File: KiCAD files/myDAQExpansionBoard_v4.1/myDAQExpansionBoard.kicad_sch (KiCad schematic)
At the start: 73 parts, among them J1 Conn_01x05_Male, J2 Conn_01x05_Male, J3 Conn_01x08_Male, J4 OSTV7XX3151, J5 Screw_Terminal_01x02, J6 Screw_Terminal_01x02, J7 Screw_Terminal_01x01, J8 Screw_Terminal_01x01, SW1 SW_SPDT, SW2 SW_SPDT, SW3 SW_Push, SW4 SW_Push, U1 74LS47, U2 7segm-symbol, U3 ACS712xLCTR-05B, U4 L298N

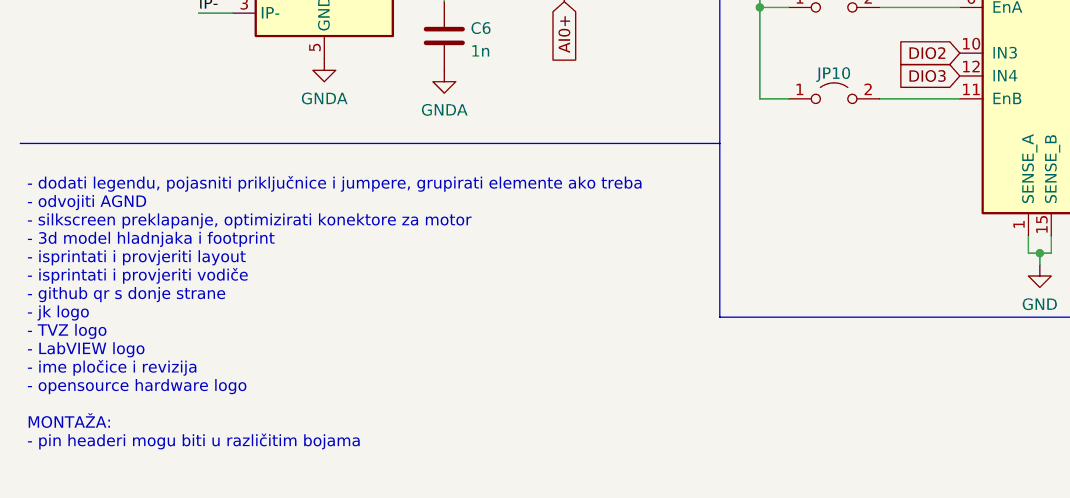
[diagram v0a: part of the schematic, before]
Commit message: update
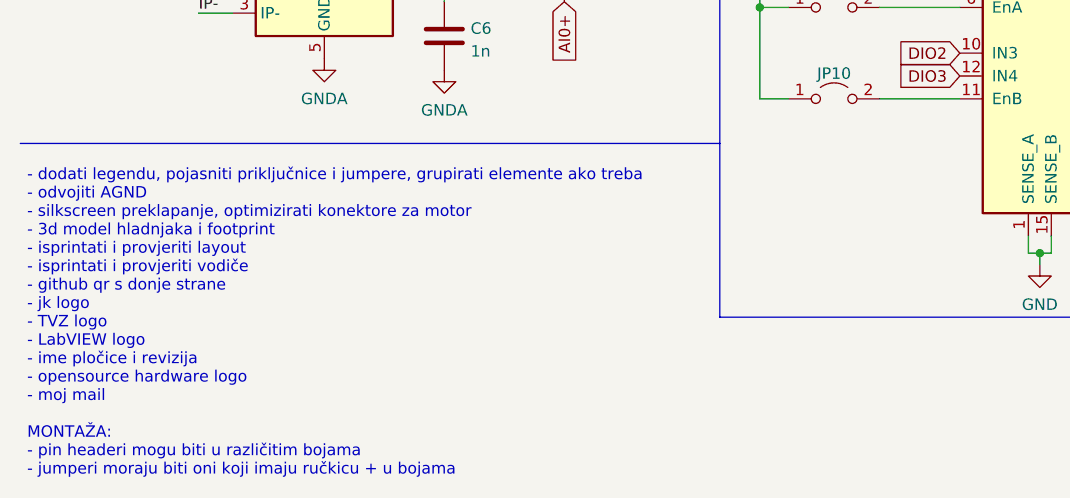
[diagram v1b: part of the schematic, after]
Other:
- note added: "- dodati legendu, pojasniti priključnice i jumpere, grupirati elemente ako treba - odvojiti AGND - silkscreen preklapanje, optimizirati konektore za motor - 3d model hladnjaka i footprint - isprintati i provjeriti layout - isprintati i provjeriti vodiče - github qr s donje strane - jk logo - TVZ logo - LabVIEW logo - ime pločice i revizija - opensource hardware logo - moj mail MONTAŽA: - pin head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"
- note removed: "- dodati legendu, pojasniti priključnice i jumpere, grupirati elemente ako treba - odvojiti AGND - silkscreen preklapanje, optimizirati konektore za motor - 3d model hladnjaka i footprint - isprintati i provjeriti layout - isprintati i provjeriti vodiče - github qr s donje strane - jk logo - TVZ logo - LabVIEW logo - ime pločice i revizija - opensource hardware logo MONTAŽA: - pin headeri mogu bi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"
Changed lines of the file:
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@@
     (effects (font (size 2 2)) (justify left bottom))
   )
-  (text "- dodati legendu, pojasniti priključnice i jumpere, grupirati elemente ako treba\n- odvojiti AGND\n- silkscreen preklapanje, optimizirati konektore za motor\n- 3d model hladnjaka i footprint\n- isprintati i provjeriti layout\n- isprintati i provjeriti vodiče\n- github qr s donje strane\n- jk logo\n- TVZ logo\n- LabVIEW logo\n- ime pločice i revizija\n- opensource hardware logo\n\nMONTAŽA:\n- pin headeri mogu biti u različitim bojama"
-    (at 12.954 187.198 0)
+  (text "- dodati legendu, pojasniti priključnice i jumpere, grupirati elemente ako treba\n- odvojiti AGND\n- silkscreen preklapanje, optimizirati konektore za motor\n- 3d model hladnjaka i footprint\n- isprintati i provjeriti layout\n- isprintati i provjeriti vodiče\n- github qr s donje strane\n- jk logo\n- TVZ logo\n- LabVIEW logo\n- ime pločice i revizija\n- opensource hardware logo\n- moj mail\n\nMONTAŽA:\n- pin headeri mogu biti u različitim bojama\n- jumperi moraju biti oni koji imaju ručkicu + u bojama"
+    (at 12.954 190.246 0)
     (effects (font (size 1.27 1.27)) (justify left bottom))
   )

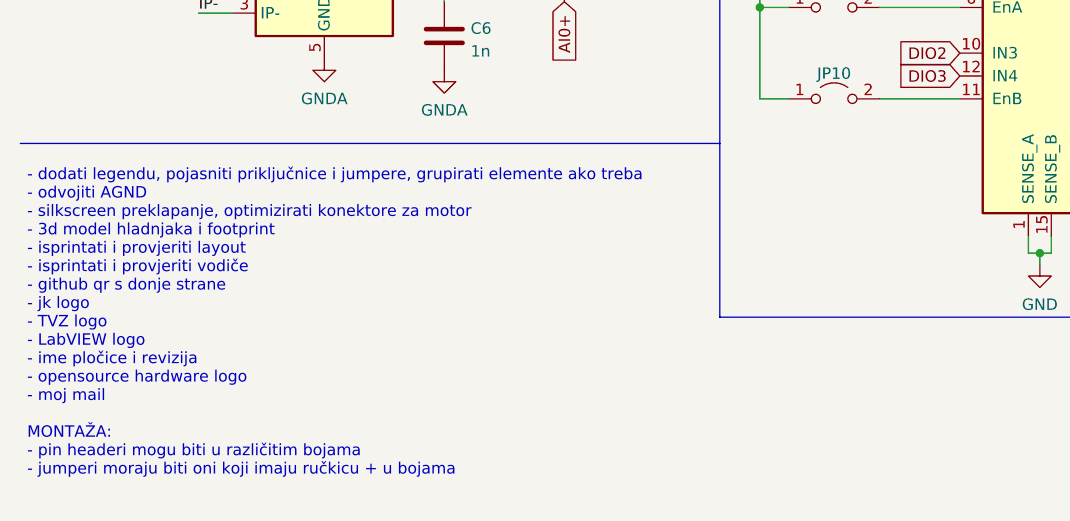
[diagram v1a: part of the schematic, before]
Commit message: update
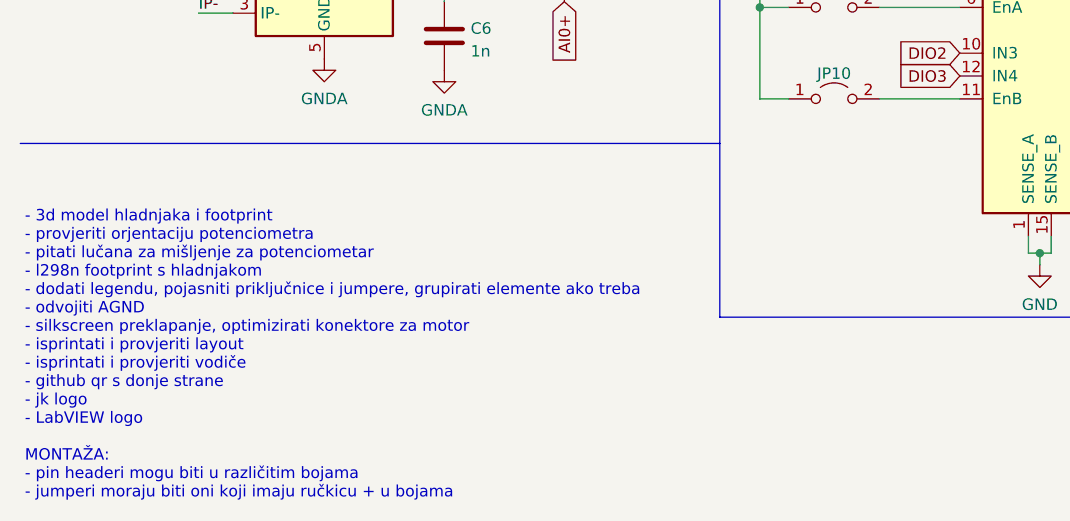
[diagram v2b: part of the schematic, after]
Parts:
- U4: footprint Library:TO-220-15_P2.54x2.54mm_StaggerOdd_Lead4.58mm_Vertical -> Library:L298n
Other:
- note added: "- 3d model hladnjaka i footprint - provjeriti orjentaciju potenciometra - pitati lučana za mišljenje za potenciometar - l298n footprint s hladnjakom - dodati legendu, pojasniti priključnice i jumpere, grupirati elemente ako treba - odvojiti AGND - silkscreen preklapanje, optimizirati konektore za motor - isprintati i provjeriti layout - isprintati i provjeriti vodiče - github qr s donje strane - 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"
- note removed: "- dodati legendu, pojasniti priključnice i jumpere, grupirati elemente ako treba - odvojiti AGND - silkscreen preklapanje, optimizirati konektore za motor - 3d model hladnjaka i footprint - isprintati i provjeriti layout - isprintati i provjeriti vodiče - github qr s donje strane - jk logo - TVZ logo - LabVIEW logo - ime pločice i revizija - opensource hardware logo - moj mail MONTAŽA: - pin head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"
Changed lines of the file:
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@@
     (effects (font (size 2 2)) (justify left bottom))
   )
-  (text "- dodati legendu, pojasniti priključnice i jumpere, grupirati elemente ako treba\n- odvojiti AGND\n- silkscreen preklapanje, optimizirati konektore za motor\n- 3d model hladnjaka i footprint\n- isprintati i provjeriti layout\n- isprintati i provjeriti vodiče\n- github qr s donje strane\n- jk logo\n- TVZ logo\n- LabVIEW logo\n- ime pločice i revizija\n- opensource hardware logo\n- moj mail\n\nMONTAŽA:\n- pin headeri mogu biti u različitim bojama\n- jumperi moraju biti oni koji imaju ručkicu + u bojama"
-    (at 12.954 190.246 0)
+  (text "- 3d model hladnjaka i footprint\n- provjeriti orjentaciju potenciometra\n- pitati lučana za mišljenje za potenciometar\n- l298n footprint s hladnjakom\n- dodati legendu, pojasniti priključnice i jumpere, grupirati elemente ako treba\n- odvojiti AGND\n- silkscreen preklapanje, optimizirati konektore za motor\n- isprintati i provjeriti layout\n- isprintati i provjeriti vodiče\n- github qr s donje strane\n- jk logo\n- LabVIEW logo\n\nMONTAŽA:\n- pin headeri mogu biti u različitim bojama\n- jumperi moraju biti oni koji imaju ručkicu + u bojama"
+    (at 12.7 192.786 0)
     (effects (font (size 1.27 1.27)) (justify left bottom))
   )
@@
       (effects (font (size 1.27 1.27)) (justify left))
     )
-    (property "Footprint" "Library:TO-220-15_P2.54x2.54mm_StaggerOdd_Lead4.58mm_Vertical" (id 2) (at 133.096 162.179 0)
+    (property "Footprint" "Library:L298n" (id 2) (at 133.096 162.179 0)
       (effects (font (size 1.27 1.27)) (justify left) hide)
     )
@@
     )
     (path "/dfb5f089-6957-4ffa-aef1-b0b311b19342"
-      (reference "U4") (unit 1) (value "L298N") (footprint "Library:TO-220-15_P2.54x2.54mm_StaggerOdd_Lead4.58mm_Vertical")
-    )
-  )
+      (reference "U4") (unit 1) (value "L298N") (footprint "Library:L298n")
+    )
+  )
